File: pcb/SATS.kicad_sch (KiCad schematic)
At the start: 15 parts, among them J1 Raspberry_Pi_2_3, SW1 SW_Reed, SW2 SW_Reed, SW3 SW_Reed, U1 MCP23017_SP, U2 MCP23017_SP, U3 CD40109BE, U4 IRLZ14PBF

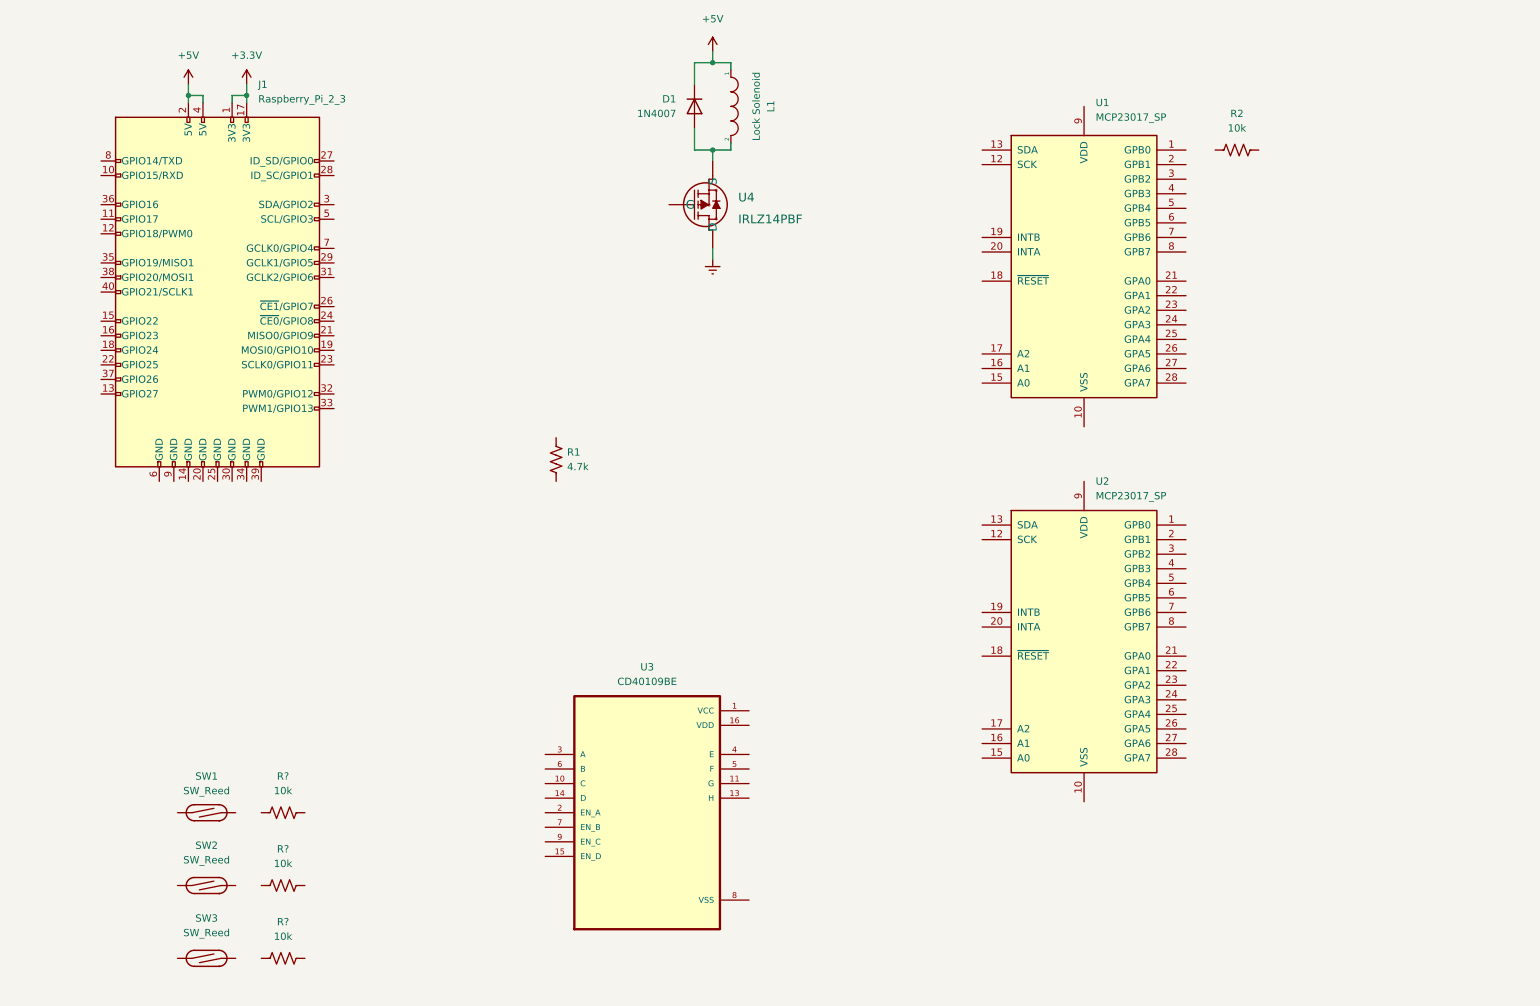
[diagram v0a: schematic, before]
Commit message: Start Net building
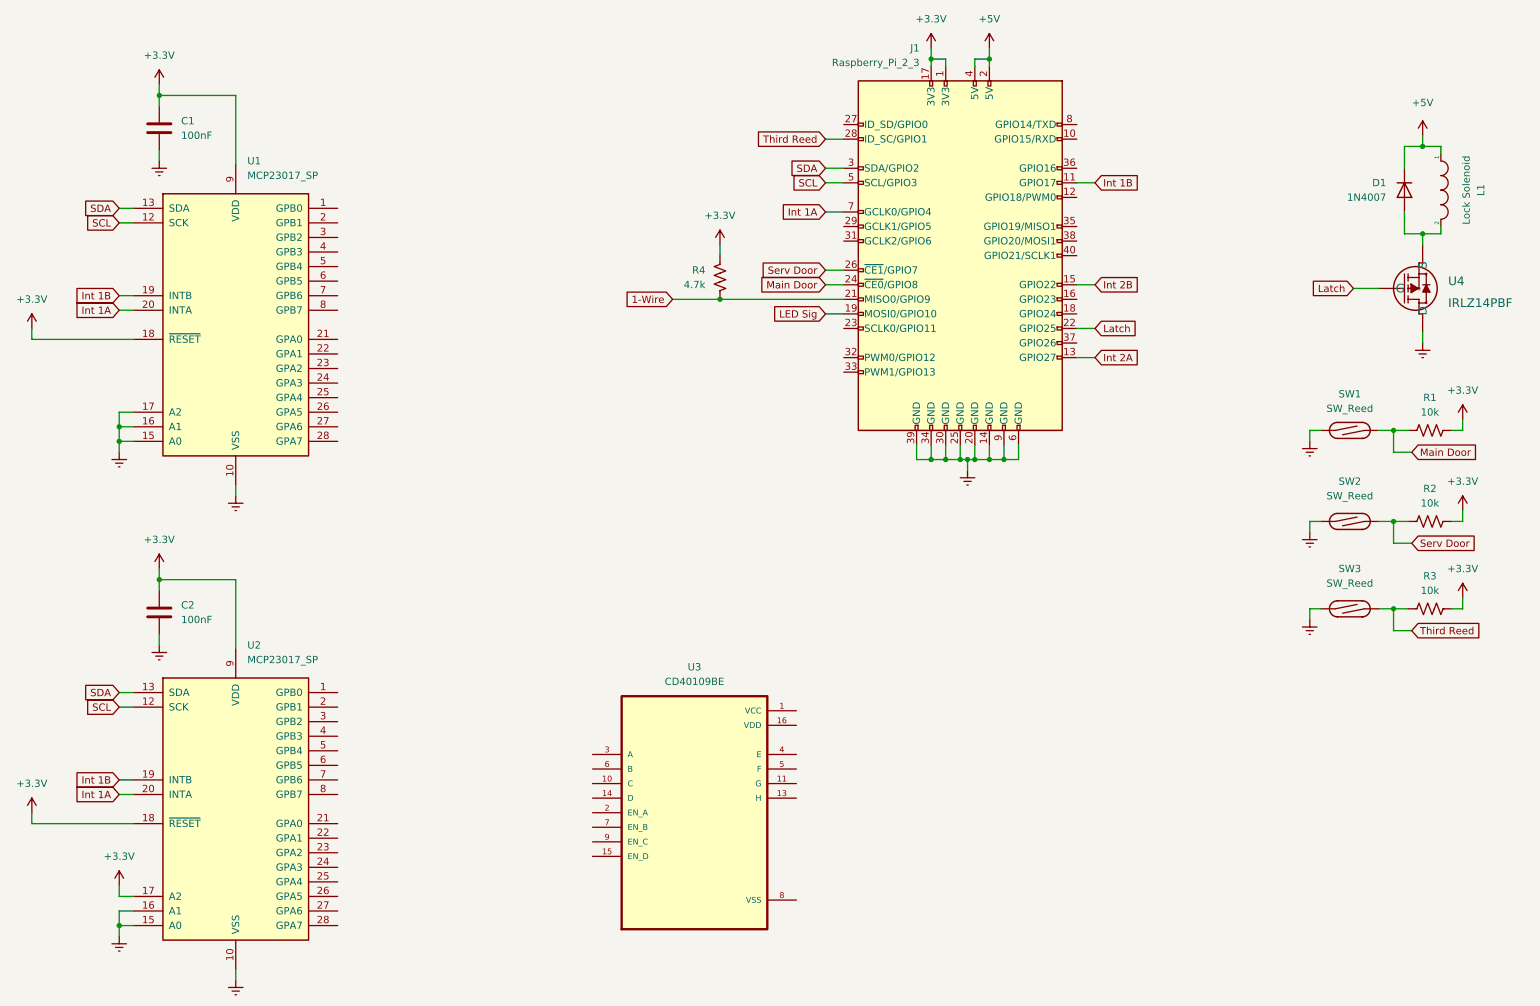
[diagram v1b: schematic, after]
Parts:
- removed R2: 10k, symbol Device:R_US
- added C1, C2: 100nF, symbol Device:C
- gave numbers to parts that had none: 3
- renumbered R1 to R4
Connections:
- net +3V3: now also R1.2, R2.2, R3.2, R4.2, U1.18 (~{RESET}), U1.9 (VDD), U2.17 (A2), U2.18 (~{RESET}), U2.9 (VDD), C1.1, C2.1
- net Earth: now also J1.14 (GND), J1.20 (GND), J1.25 (GND), J1.30 (GND), J1.34 (GND), J1.39 (GND), J1.6 (GND), J1.9 (GND), SW1.1, SW2.1, SW3.1, U1.10 (VSS), U1.15 (A0), U1.16 (A1), U1.17 (A2), U2.10 (VSS), U2.15 (A0), U2.16 (A1), C1.2, C2.2
- net Third Reed: now reaches R3.1
- net Third Reed: now also J1.28 (ID_SC/GPIO1), SW3.2
- net SCL: now reaches U1.12 (SCK)
- net SCL: now also J1.5 (SCL/GPIO3), U2.12 (SCK)
- net SDA: now reaches U1.13 (SDA)
- net SDA: now also J1.3 (SDA/GPIO2), U2.13 (SDA)
- net Int 1B: now reaches U1.19 (INTB)
- net Int 1B: now also J1.11 (GPIO17), U2.19 (INTB)
- net Int 1A: now reaches U1.20 (INTA)
- net Int 1A: now also J1.7 (GCLK0/GPIO4), U2.20 (INTA)
- net Main Door: now reaches R1.1
- net Main Door: now also J1.24 (~{CE0}/GPIO8), SW1.2
- net Serv Door: now reaches R2.1
- net Serv Door: now also J1.26 (~{CE1}/GPIO7), SW2.2
- net Int 2A: now reaches J1.13 (GPIO27)
- net Int 2B: now reaches J1.15 (GPIO22)
- net LED Sig: now reaches J1.19 (MOSI0/GPIO10)
- net 1-Wire: now reaches J1.21 (MISO0/GPIO9)
- net 1-Wire: now also R4.1
- net Latch: now reaches J1.22 (GPIO25)
- net Latch: now also U4.1 (G)
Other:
- moved on the sheet: D1, J1, L1, R1, R2, R3, R4, SW1, SW2, SW3, U1, U3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
